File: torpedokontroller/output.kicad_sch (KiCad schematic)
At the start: 34 parts, among them IC1 NCP81296MNTXG, IC9 TCAN3414DR, J1 64900411122, J7 H, J8 L, Q1 STANDARD_140356145200, Q2 SiS443DN, Q6 PMOS

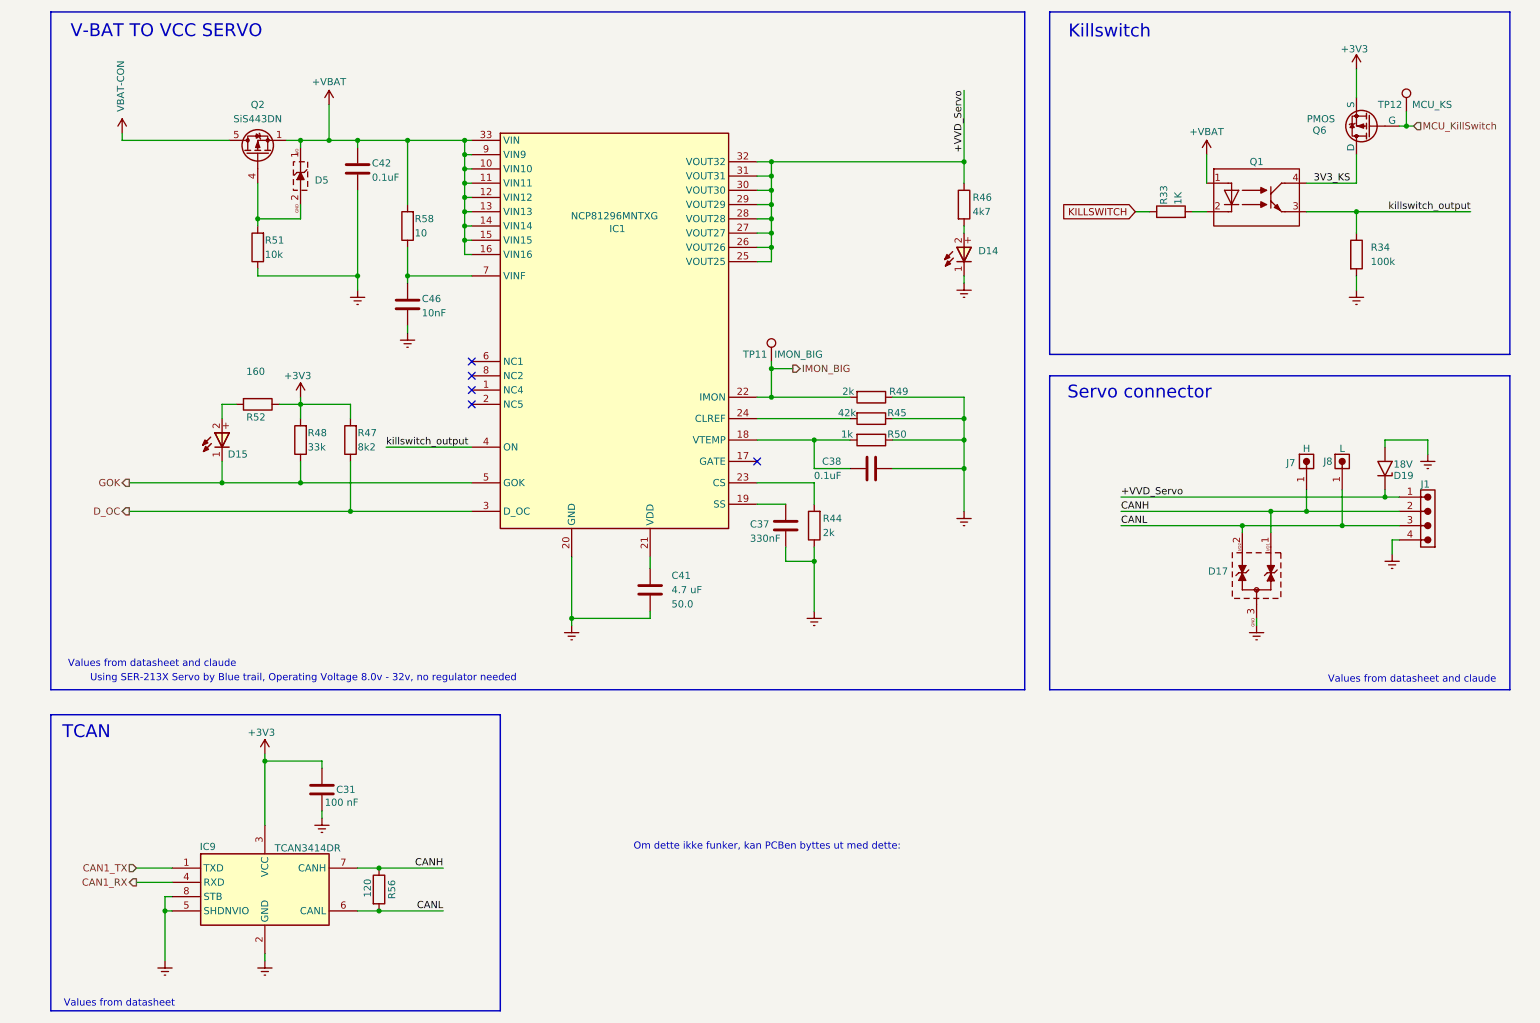
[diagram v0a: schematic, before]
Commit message: v 1.2
PWM SERVOS :)) YAAADDAAAAAa
Layout begynner å komme seg
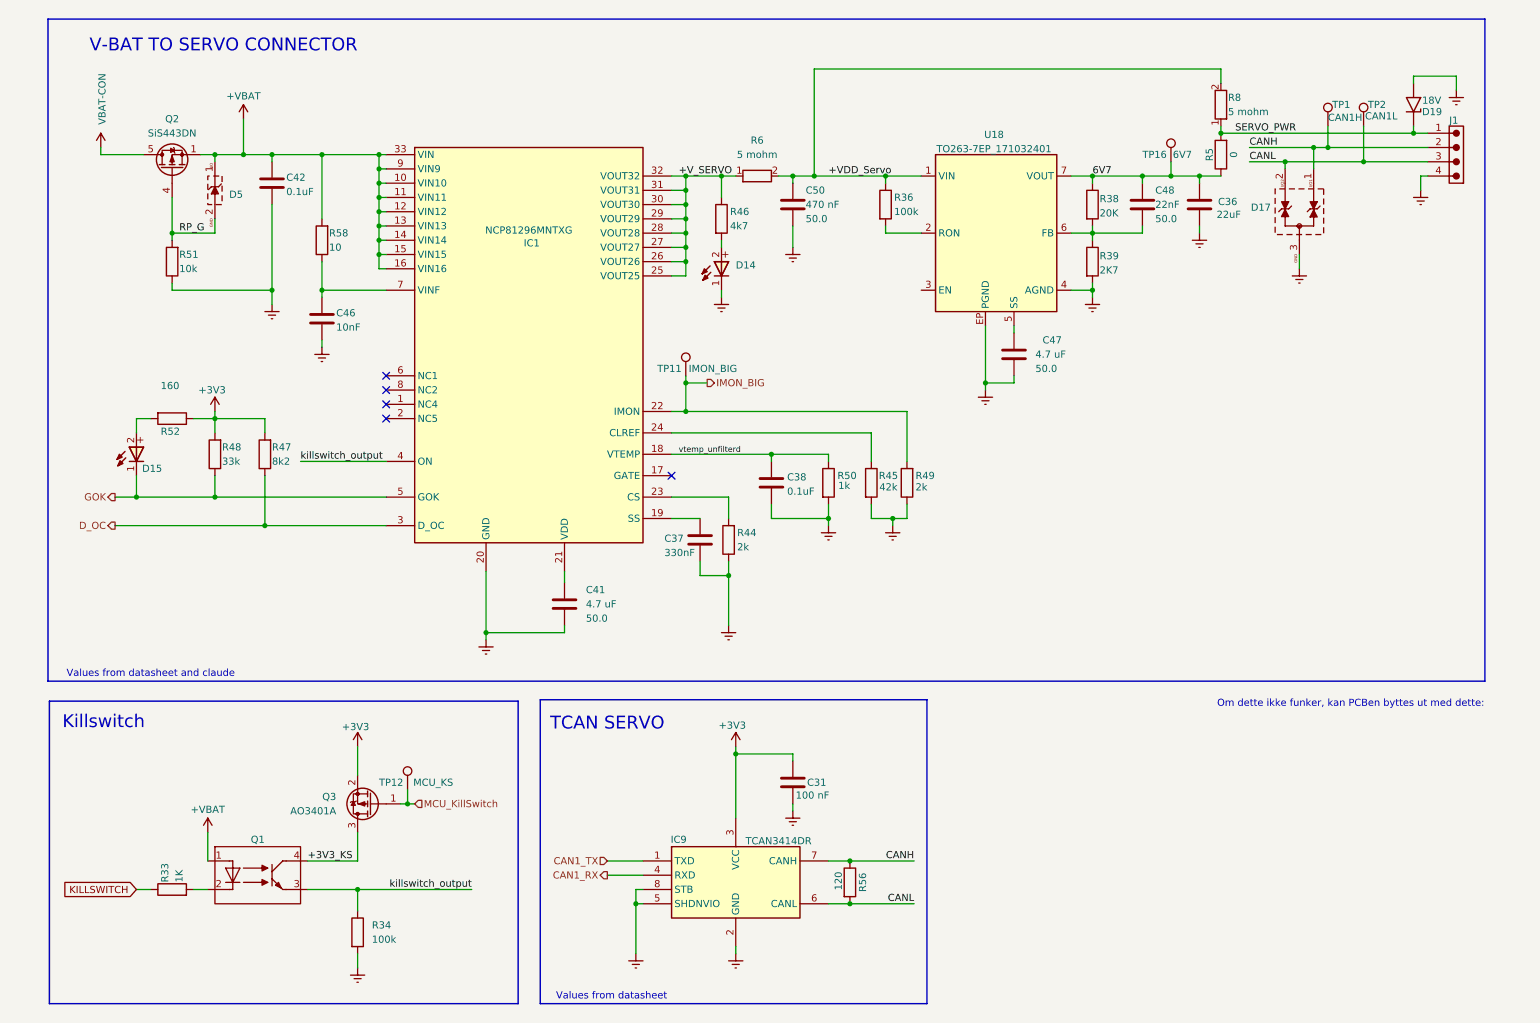
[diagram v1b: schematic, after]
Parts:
- removed J7: H, Connectors_tht:J_Wurth_WR-PHD_61300111121, symbol Connector_Wurth_WR-PHD:61300111121
- removed J8: L, Connectors_tht:J_Wurth_WR-PHD_61300111121, symbol Connector_Wurth_WR-PHD:61300111121
- removed Q6: PMOS, symbol Simulation_SPICE:PMOS
- added C36: 22uF, Capasitors:C_Wurth_WCAP-CSGP-0603_R, symbol Capacitor_Wurth_WCAP-CSGP:1210_H2.5_885012209048
- added C47: 4.7 uF, Capasitors:C_Wurth_WCAP-CSGP-0603_R, symbol Capacitor_Wurth_WCAP-CSGP:1210_H2.5_885012209048
- added C48: 22nF, Capasitors:C_Wurth_WCAP-CSGP-0603_R, symbol Capacitor_Wurth_WCAP-CSGP:1210_H2.5_885012209048
- added C50: 470 nF, Capasitors:C_Wurth_WCAP-CSGP-0603_R, symbol Capacitor_Wurth_WCAP-CSGP:1210_H2.5_885012209048
- added Q3: AO3401A, Package_TO_SOT_SMD:SOT-23, symbol Transistor_FET:AO3401A
- added R36: 100k, WE-Resistors:R_Wurth_WRIS-KSKE-0603, symbol Device:R
- added R38: 20K, WE-Resistors:R_Wurth_WRIS-KSKE-0603, symbol Device:R
- added R39: 2K7, WE-Resistors:R_Wurth_WRIS-KSKE-0603, symbol Device:R
- added R5: 0, WE-Resistors:R_Wurth_WRIS-KSKE-0603, symbol Device:R
- added R6, R8: 5 mohm, Resistor_SMD_Wurth:R_Wurth_WRIS-PSMC-2512_L6.3W3.1H0.51, symbol WRIS-PSMC:2512_L6.3W3.1H0.51_580070763005
- added TP1: CAN1H, TestPoint:TestPoint_Keystone_5000-5004_Miniature, symbol Connector:TestPoint
- added TP16: TestPoint, TestPoint:TestPoint_Pad_D1.5mm, symbol Connector:TestPoint
- added TP2: CAN1L, TestPoint:TestPoint_Keystone_5000-5004_Miniature, symbol Connector:TestPoint
- added U18: TO263-7EP_171032401, MagIC_SMD_Wurth:U_Wurth_WPME-VDRM-TO263-7EP, symbol WR-VDRM:TO263-7EP_171032401
- D5: footprint Diode_SMD_Wurth:D_Wurth_WE-TVS-DFN1610-2L -> zener:824045817
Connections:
- net +3V3: now also Q3.2 (S)
- net CANH: now also TP1.1
- net CANL: now also TP2.1
- net Earth: now also R45.2, R50.2, C36.2, C47.2, C50.2, R39.2, U18.4 (AGND), U18.EP (PGND); no longer R45.1, R50.1
- net MCU_KillSwitch: now also Q3.1 (G)
- net at IC1.24 (CLREF): now also R45.1; no longer R45.2
- net RP_G: now reaches D5.2 (GND), Q2.4 (G), R51.2
- net vtemp_unfilterd: now reaches C38.1, IC1.18 (VTEMP)
- net vtemp_unfilterd: now also R50.1; no longer R50.2
- net +VVD_Servo renamed +V_SERVO
- net +V_SERVO: now also R6.1; no longer D19.1 (A1), J1.1
- net 3V3_KS renamed +3V3_KS
- net +3V3_KS: now also Q3.3 (D)
- new net: C48.2, R38.2, R39.1, U18.6 (FB)
- new net: R36.2, U18.2 (RON)
- new net: C47.1, U18.5 (SS)
- new net +VDD_Servo: C50.1, R36.1, R6.2, R8.2, U18.1 (VIN)
- new net 6V7: C36.1, C48.1, R38.1, R5.1, TP16.1, U18.7 (VOUT)
- new net SERVO_PWR: D19.1 (A1), J1.1, R5.2, R8.1
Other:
- note added: "TCAN SERVO"
- note added: "V-BAT TO SERVO CONNECTOR"
- note removed: "Servo connector"
- note removed: "TCAN"
- note removed: "Using SER-213X Servo by Blue trail, Operating Voltage 8.0v - 32v, no regulator needed"
- note removed: "V-BAT TO VCC SERVO"
- moved on the sheet: C31, C37, C38, C41, C42, C46, D14, D15, D17, D19, D5, IC1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
